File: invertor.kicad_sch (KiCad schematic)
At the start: 6 parts, among them IC401 BD33IA5WEFJ-E2, T401 FS10-250

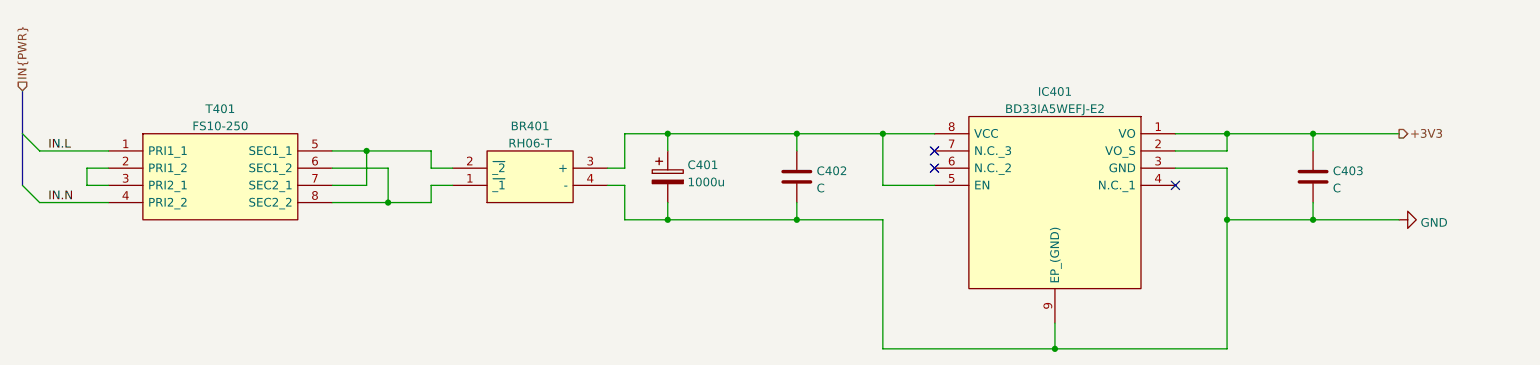
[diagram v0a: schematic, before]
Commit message: Schematic cleanup
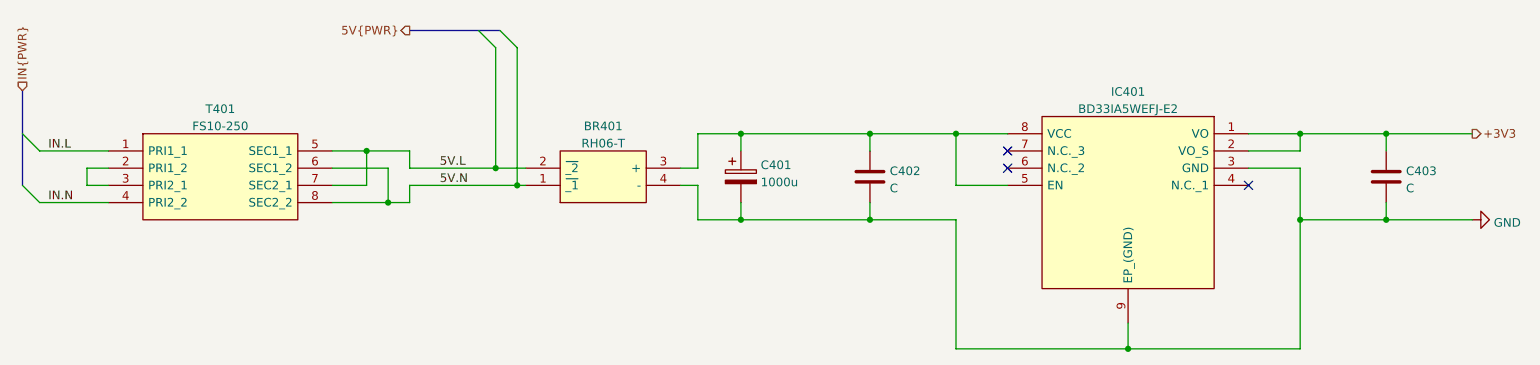
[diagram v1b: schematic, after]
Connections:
- net 5V.N: now reaches BR401.1 (~{_1}), T401.6 (SEC1_2), T401.8 (SEC2_2)
- net 5V.L: now reaches BR401.2 (~{_2}), T401.5 (SEC1_1), T401.7 (SEC2_1)
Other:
- moved on the sheet: BR401, C401, C402, C403, IC401
